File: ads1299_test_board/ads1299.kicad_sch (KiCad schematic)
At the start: 26 parts, among them CN1 W2A45C103MAT2A, CN2 W2A45C103MAT2A, J3 Conn_02x05_Top_Bottom, U1 ADS1299, U4 OPA376xxD

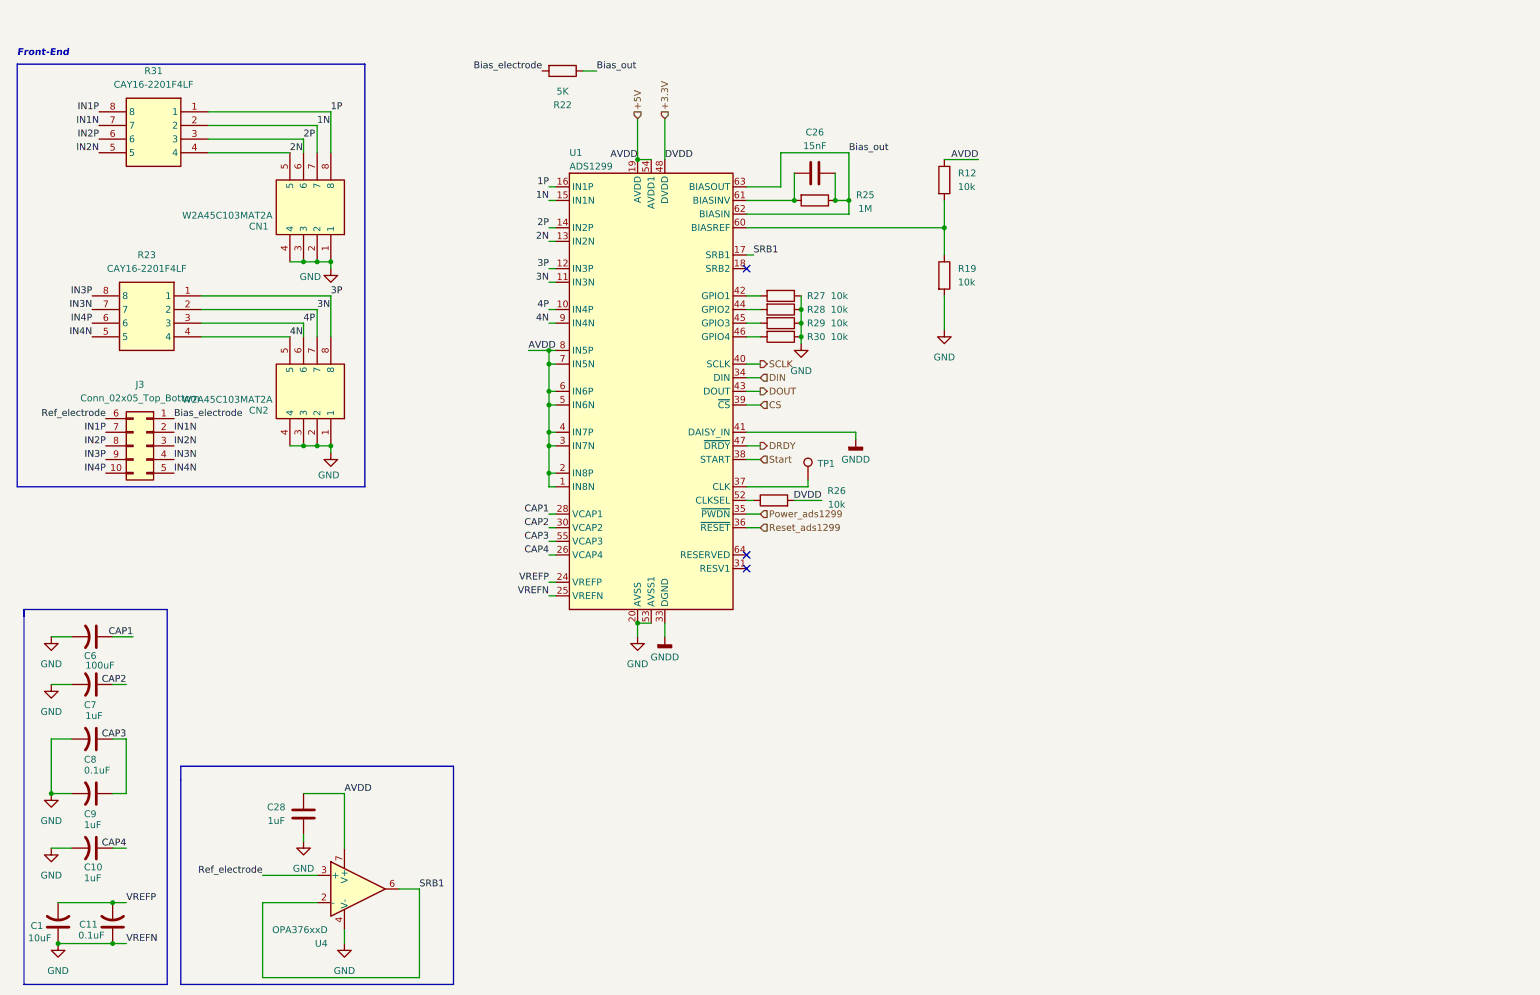
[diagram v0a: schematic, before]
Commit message: 8 channel
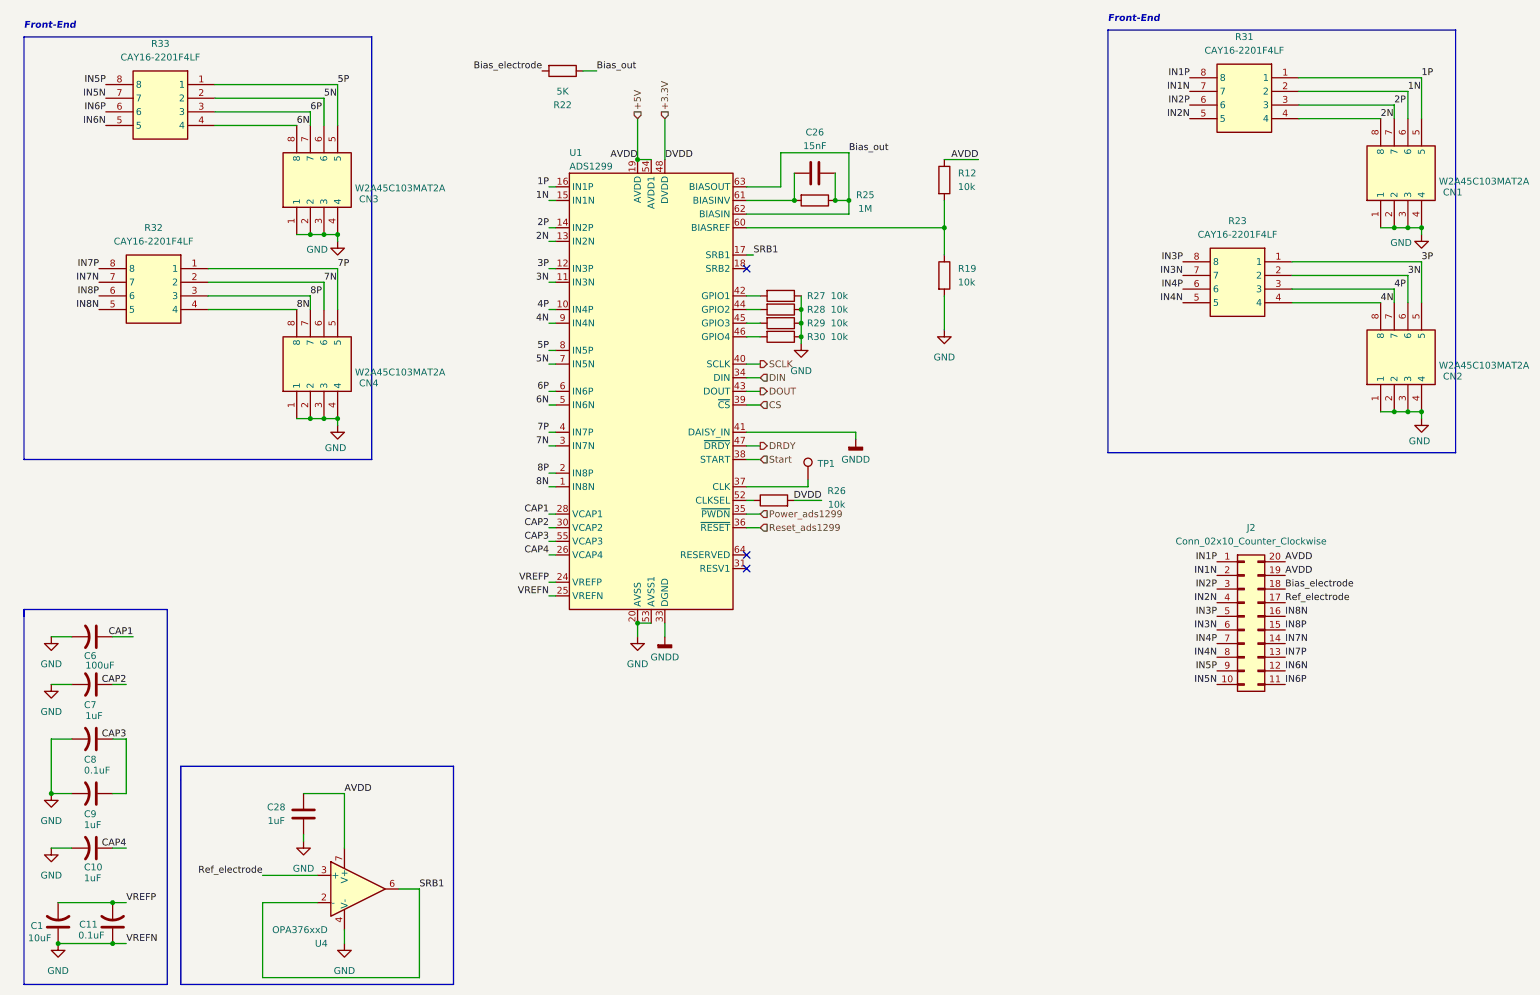
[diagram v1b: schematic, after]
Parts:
- removed J3: Conn_02x05_Top_Bottom, Connector_Molex:Molex_Mini-Fit_Jr_5566-10A_2x05_P4.20mm_Vertical, symbol Connector_Generic:Conn_02x05_Top_Bottom
- added CN3, CN4: W2A45C103MAT2A, W2A45C103MAT2A:W2A45C103MAT2A, symbol W2A45C103MAT2A:W2A45C103MAT2A
- added J2: Conn_02x10_Counter_Clockwise, Connector_IDC:IDC-Header_2x10_P2.54mm_Vertical, symbol Connector_Generic:Conn_02x10_Counter_Clockwise
- added R32, R33: CAY16-2201F4LF, CAY16-2201F4LF:RESCAX80P160X320X60-8N, symbol CAY16-2201F4LF:CAY16-2201F4LF
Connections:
- net +5V: now also J2.19 (Pin_19), J2.20 (Pin_20); no longer U1.1 (IN8N), U1.2 (IN8P), U1.3 (IN7N), U1.4 (IN7P), U1.5 (IN6N), U1.6 (IN6P), U1.7 (IN5N), U1.8 (IN5P)
- net 1N: now also CN1.6; no longer CN1.7
- net 1P: now also CN1.5; no longer CN1.8
- net 2N: now also CN1.8; no longer CN1.5
- net 2P: now also CN1.7; no longer CN1.6
- net 3N: now also CN2.6; no longer CN2.7
- net 3P: now also CN2.5; no longer CN2.8
- net 4N: now also CN2.8; no longer CN2.5
- net 4P: now also CN2.7; no longer CN2.6
- net Bias_electrode: now also J2.18 (Pin_18)
- net GND: now also CN3.1, CN3.2, CN3.3, CN3.4, CN4.1, CN4.2, CN4.3, CN4.4
- net IN1N: now also J2.2 (Pin_2)
- net IN1P: now also J2.1 (Pin_1)
- net IN2N: now also J2.4 (Pin_4)
- net IN2P: now also J2.3 (Pin_3)
- net IN3N: now also J2.6 (Pin_6)
- net IN3P: now also J2.5 (Pin_5)
- net IN4N: now also J2.8 (Pin_8)
- net IN4P: now also J2.7 (Pin_7)
- net Ref_electrode: now also J2.17 (Pin_17)
- new net 5N: CN3.6, R33.2, U1.7 (IN5N)
- new net 5P: CN3.5, R33.1, U1.8 (IN5P)
- new net 6N: CN3.8, R33.4, U1.5 (IN6N)
- new net 6P: CN3.7, R33.3, U1.6 (IN6P)
- new net 7N: CN4.6, R32.2, U1.3 (IN7N)
- new net 7P: CN4.5, R32.1, U1.4 (IN7P)
- new net 8N: CN4.8, R32.4, U1.1 (IN8N)
- new net 8P: CN4.7, R32.3, U1.2 (IN8P)
- new net IN5N: J2.10 (Pin_10), R33.7
- new net IN5P: J2.9 (Pin_9), R33.8
- new net IN6N: J2.12 (Pin_12), R33.5
- new net IN6P: J2.11 (Pin_11), R33.6
- new net IN7N: J2.14 (Pin_14), R32.7
- new net IN7P: J2.13 (Pin_13), R32.8
- new net IN8N: J2.16 (Pin_16), R32.5
- new net IN8P: J2.15 (Pin_15), R32.6
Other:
- moved on the sheet: CN1, CN2, R23, R31
